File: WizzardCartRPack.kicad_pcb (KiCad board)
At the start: 2 copper layers, 72.7 x 54.5 mm, 6 parts, among them SW1 SW_SPDT, U2 27C512

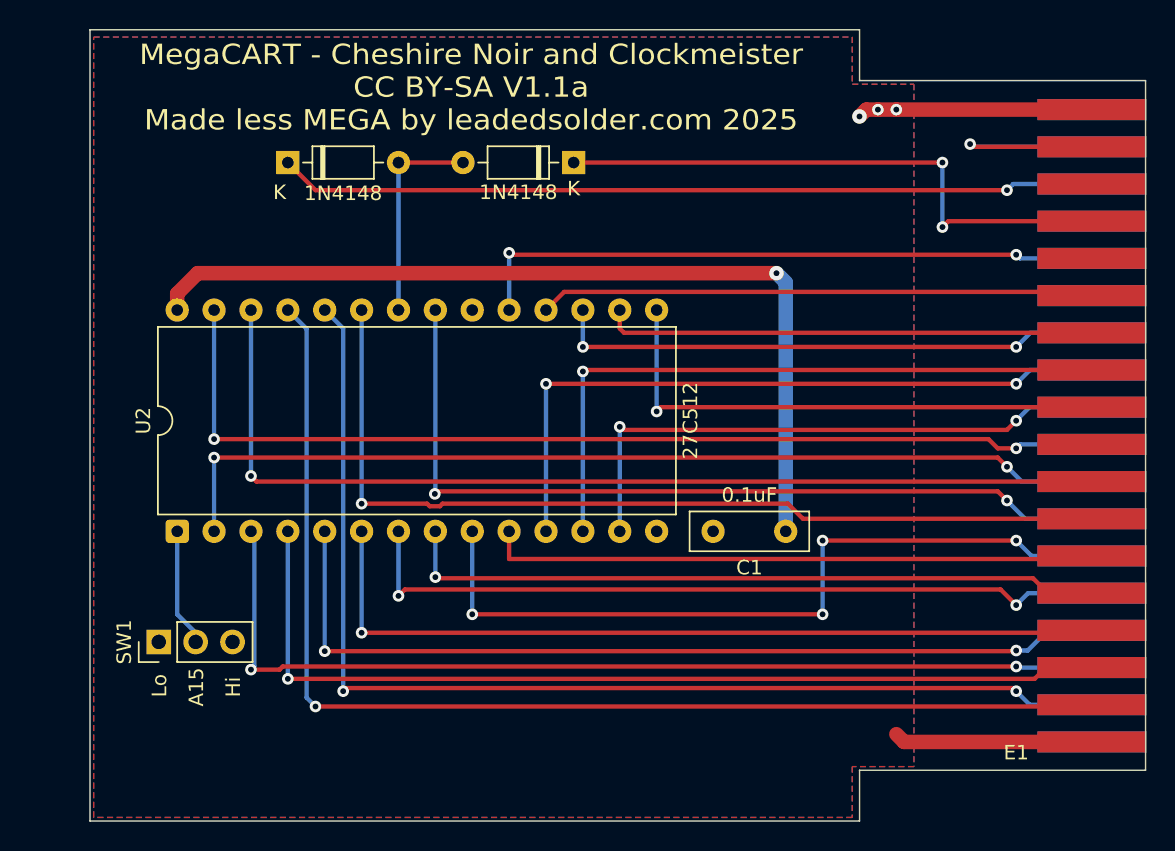
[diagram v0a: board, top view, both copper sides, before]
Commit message: Move fingers up
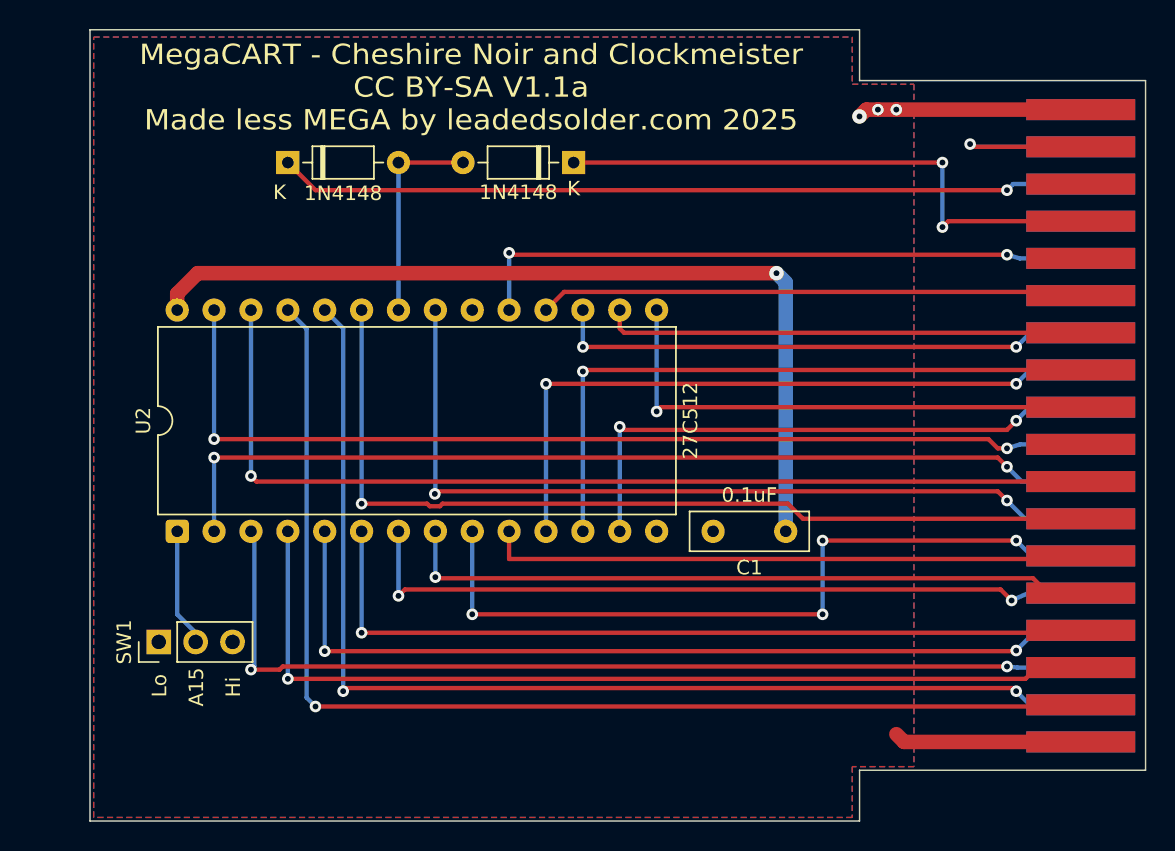
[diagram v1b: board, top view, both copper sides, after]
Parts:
- moved E1 0.76 mm to (159.7, 120.5)
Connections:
- net Net-(D1-A) renamed /~{OE}
- net Net-(D1-K) renamed /~{ROM1}
- net Net-(D2-K) renamed /~{ROM2}
- net Net-(SW1-B) renamed /A15
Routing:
- net /A6: track 65.9 -> 68.3 mm
- net /A5: track 61.7 -> 63.9 mm
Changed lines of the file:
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@@
 	(net 1 "GND")
 	(net 2 "+5V")
-	(net 3 "Net-(D1-K)")
-	(net 4 "Net-(D1-A)")
-	(net 5 "Net-(D2-K)")
+	(net 3 "/~{ROM1}")
+	(net 4 "/~{OE}")
+	(net 5 "/~{ROM2}")
 	(net 6 "/A1")
 	(net 7 "/A10")
@@
 	(net 35 "/A7")
 	(net 36 "unconnected-(E1-PHI2-Pad26)")
-	(net 37 "Net-(SW1-B)")
+	(net 37 "/A15")
 	(footprint "Diode_THT:D_DO-35_SOD27_P7.62mm_Horizontal"
 		(layer "F.Cu")
@@
 			(layers "*.Cu" "*.Mask")
 			(remove_unused_layers no)
-			(net 5 "Net-(D2-K)")
+			(net 5 "/~{ROM2}")
 			(pinfunction "K")
 			(pintype "passive")
@@
 			(layers "*.Cu" "*.Mask")
 			(remove_unused_layers no)
-			(net 4 "Net-(D1-A)")
+			(net 4 "/~{OE}")
 			(pinfunction "A")
 			(pintype "passive")
@@
 	(footprint "WizzardCart:36Edge"
 		(layer "F.Cu")
-		(at 160.5 120.55 90)
+		(at 159.735 120.55 90)
 		(property "Reference" "E1"
 			(at -0.735 0.79 180)
 			(layer "F.SilkS")
+			(hide yes)
 			(effects
 				(font
@@
 			(size 1.45 7.5)
 			(layers "F.Cu" "F.Mask")
-			(net 3 "Net-(D1-K)")
+			(net 3 "/~{ROM1}")
 			(pinfunction "_ROM1")
 			(pintype "bidirectional")
@@
 			(size 1.45 7.5)
 			(layers "B.Cu" "B.Mask")
-			(net 5 "Net-(D2-K)")
+			(net 5 "/~{ROM2}")
 			(pinfunction "_ROM2")
 			(pintype "bidirectional")
@@
 			(layers "*.Cu" "*.Mask")
 			(remove_unused_layers no)
-			(net 3 "Net-(D1-K)")
+			(net 3 "/~{ROM1}")
 			(pinfunction "K")
 			(pintype "passive")
@@
 			(layers "*.Cu" "*.Mask")
 			(remove_unused_layers no)
-			(net 4 "Net-(D1-A)")
+			(net 4 "/~{OE}")
 			(pinfunction "A")
 			(pintype "passive")
@@
 			(layers "*.Cu" "*.Mask")
 			(remove_unused_layers no)
-			(net 37 "Net-(SW1-B)")
+			(net 37 "/A15")
 			(pinfunction "B")
 			(pintype "passive")
@@
 			(remove_unused_layers no)
 			(roundrect_rratio 0.15625)
-			(net 37 "Net-(SW1-B)")
+			(net 37 "/A15")
 			(pinfunction "A15")
 			(pintype "input")
@@
 			(layers "*.Cu" "*.Mask")
 			(remove_unused_layers no)
-			(net 4 "Net-(D1-A)")
+			(net 4 "/~{OE}")
 			(pinfunction "~{OE}")
 			(pintype "input")
@@
 	)
 	(segment
-		(start 161.29 86.995)
+		(start 160.655 86.995)
 		(end 126.495 86.995)
 		(width 0.3)
@@
 	)
 	(via
-		(at 161.29 86.995)
+		(at 160.655 86.995)
 		(size 0.8)
 		(drill 0.4)
@@
 	)
 	(segment
-		(start 161.542068 87.247068)
-		(end 161.29 86.995)
+		(start 126.365 90.805)
+		(end 126.365 86.865)
 		(width 0.3)
 		(layer "B.Cu")
@@
 	)
 	(segment
-		(start 126.365 90.805)
-		(end 126.365 86.865)
+		(start 160.655 86.995)
+		(end 161.542068 87.247068)
 		(width 0.3)
 		(layer "B.Cu")
@@
 	)
 	(segment
-		(start 166.5 87.247068)
-		(end 161.542068 87.247068)
+		(start 161.542068 87.247068)
+		(end 166.5 87.247068)
 		(width 0.3)
 		(layer "B.Cu")
@@
 		(net 13)
 	)
-	(segment
-		(start 166.5 112.864708)
-		(end 166.334708 113.03)
-		(width 0.3)
-		(layer "F.Cu")
-		(net 13)
-	)
 	(via
 		(at 116.205 113.03)
@@
 	)
 	(segment
-		(start 166.5 89.808832)
-		(end 166.245168 89.554)
-		(width 0.3)
-		(layer "F.Cu")
-		(net 14)
-	)
-	(segment
 		(start 130.156 89.554)
 		(end 128.905 90.805)
@@
 	)
 	(segment
-		(start 163.475 112.864708)
-		(end 162.084711 114.254997)
+		(start 162.680289 112.864708)
+		(end 165.735 112.864708)
 		(width 0.3)
 		(layer "B.Cu")
@@
 	)
 	(segment
-		(start 162.084711 114.254997)
-		(end 161.29 114.254997)
+		(start 161.29 114.254997)
+		(end 162.680289 112.864708)
 		(width 0.3)
 		(layer "B.Cu")
@@
 	)
 	(segment
-		(start 161.29 111.125)
-		(end 160.214 110.049)
+		(start 160.214 110.049)
+		(end 119.186 110.049)
 		(width 0.3)
 		(layer "F.Cu")
@@
 	)
 	(segment
-		(start 119.186 110.049)
-		(end 118.745 110.49)
+		(start 160.9725 110.8075)
+		(end 160.214 110.049)
 		(width 0.3)
 		(layer "F.Cu")
@@
 	)
 	(segment
-		(start 160.214 110.049)
-		(end 119.186 110.049)
+		(start 119.186 110.049)
+		(end 118.745 110.49)
 		(width 0.3)
 		(layer "F.Cu")
@@
 	)
 	(via
-		(at 161.29 111.125)
+		(at 160.9725 110.8075)
 		(size 0.8)
 		(drill 0.4)
@@
 	)
 	(segment
-		(start 166.5 110.302944)
-		(end 162.112056 110.302944)
+		(start 162.112056 110.302944)
+		(end 166.5 110.302944)
 		(width 0.3)
 		(layer "B.Cu")
@@
 	)
 	(segment
-		(start 162.112056 110.302944)
-		(end 161.29 111.125)
+		(start 160.9725 110.8075)
+		(end 162.112056 110.302944)
 		(width 0.3)
 		(layer "B.Cu")
@@
 		(net 23)
 	)
-	(segment
-		(start 166.5 117.988236)
-		(end 166.378236 118.11)
-		(width 0.3)
-		(layer "F.Cu")
-		(net 23)
-	)
 	(via
 		(at 113.03 118.11)
@@
 	)
 	(segment
-		(start 160.02 100.33)
-		(end 159.385 99.695)
+		(start 159.385 99.695)
+		(end 106.045 99.695)
 		(width 0.3)
 		(layer "F.Cu")
@@
 	)
 	(segment
-		(start 161.29 100.33)
-		(end 160.02 100.33)
+		(start 160.02 100.33)
+		(end 159.385 99.695)
 		(width 0.3)
 		(layer "F.Cu")
@@
 	)
 	(segment
-		(start 159.385 99.695)
-		(end 106.045 99.695)
+		(start 160.655 100.33)
+		(end 160.02 100.33)
 		(width 0.3)
 		(layer "F.Cu")
@@
 	)
 	(via
-		(at 161.29 100.33)
+		(at 160.655 100.33)
 		(size 0.8)
 		(drill 0.4)
@@
 	)
 	(segment
-		(start 161.564112 100.055888)
-		(end 161.29 100.33)
+		(start 160.655 100.33)
+		(end 161.564112 100.055888)
 		(width 0.3)
 		(layer "B.Cu")
@@
 	)
 	(segment
-		(start 166.5 100.055888)
-		(end 161.564112 100.055888)
+		(start 106.045 99.695)
+		(end 106.045 90.805)
 		(width 0.3)
 		(layer "B.Cu")
@@
 	)
 	(segment
-		(start 106.045 99.695)
-		(end 106.045 90.805)
+		(start 161.564112 100.055888)
+		(end 166.5 100.055888)
 		(width 0.3)
 		(layer "B.Cu")
@@
 	)
 	(segment
-		(start 163.338528 115.426472)
-		(end 162.56 116.205)
+		(start 162.703528 115.426472)
+		(end 161.925 116.205)
+		(width 0.3)
+		(layer "F.Cu")
+		(net 31)
+	)
+	(segment
+		(start 161.925 116.205)
+		(end 111.125 116.205)
 		(width 0.3)
 		(layer "F.Cu")
@@
 	)
 	(segment
-		(start 162.56 116.205)
-		(end 111.125 116.205)
+		(start 165.735 115.426472)
+		(end 162.703528 115.426472)
 		(width 0.3)
 		(layer "F.Cu")
@@
 	)
 	(segment
-		(start 166.5 107.74118)
-		(end 166.29118 107.95)
-		(width 0.3)
-		(layer "F.Cu")
-		(net 33)
-	)
-	(segment
 		(start 166.29118 107.95)
 		(end 126.365 107.95)
@@
 	)
 	(segment
-		(start 110.557918 115.57)
+		(start 160.655 115.355)
 		(end 110.772918 115.355)
 		(width 0.3)
@@
 	(segment
 		(start 110.772918 115.355)
-		(end 161.29 115.355)
+		(end 110.557918 115.57)
 		(width 0.3)
 		(layer "F.Cu")
@@
 	)
 	(segment
-		(start 108.585 115.57)
-		(end 110.557918 115.57)
+		(start 110.557918 115.57)
+		(end 108.585 115.57)
 		(width 0.3)
 		(layer "F.Cu")
@@
 	)
 	(via
-		(at 161.29 115.355)
+		(at 160.655 115.355)
 		(size 0.8)
 		(drill 0.4)
@@
 	)
 	(segment
-		(start 166.5 115.426472)
+		(start 160.655 115.355)
 		(end 161.361472 115.426472)
 		(width 0.3)
@@
 	(segment
 		(start 161.361472 115.426472)
-		(end 161.29 115.355)
+		(end 166.5 115.426472)
 		(width 0.3)
 		(layer "B.Cu")
